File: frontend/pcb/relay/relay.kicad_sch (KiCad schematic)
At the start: 17 parts, among them J1 Conn_01x02, J2 Conn_01x02, J3 CONN_01X02, J4 Conn_01x02, K1 G6B-1114C-US5DC, Q3 BSS138, U2 DSN-MINI-360

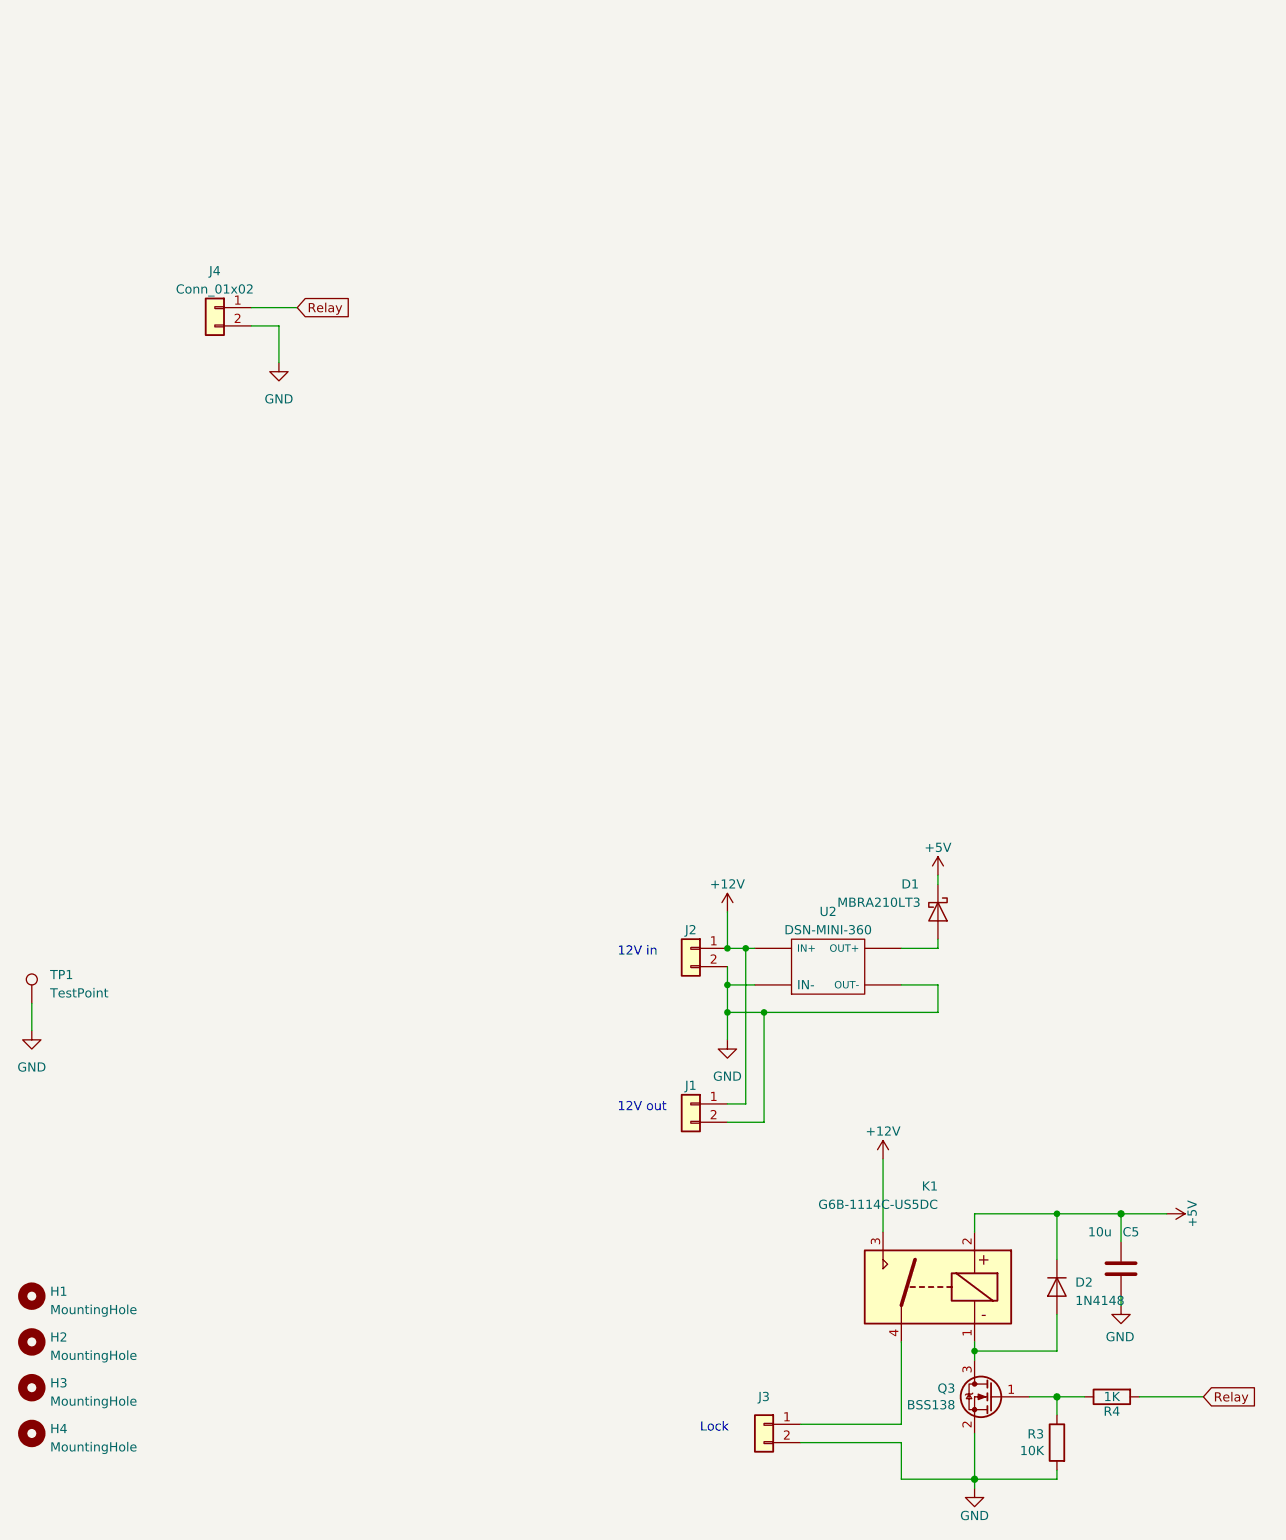
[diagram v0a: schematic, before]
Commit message: Finish relay board.
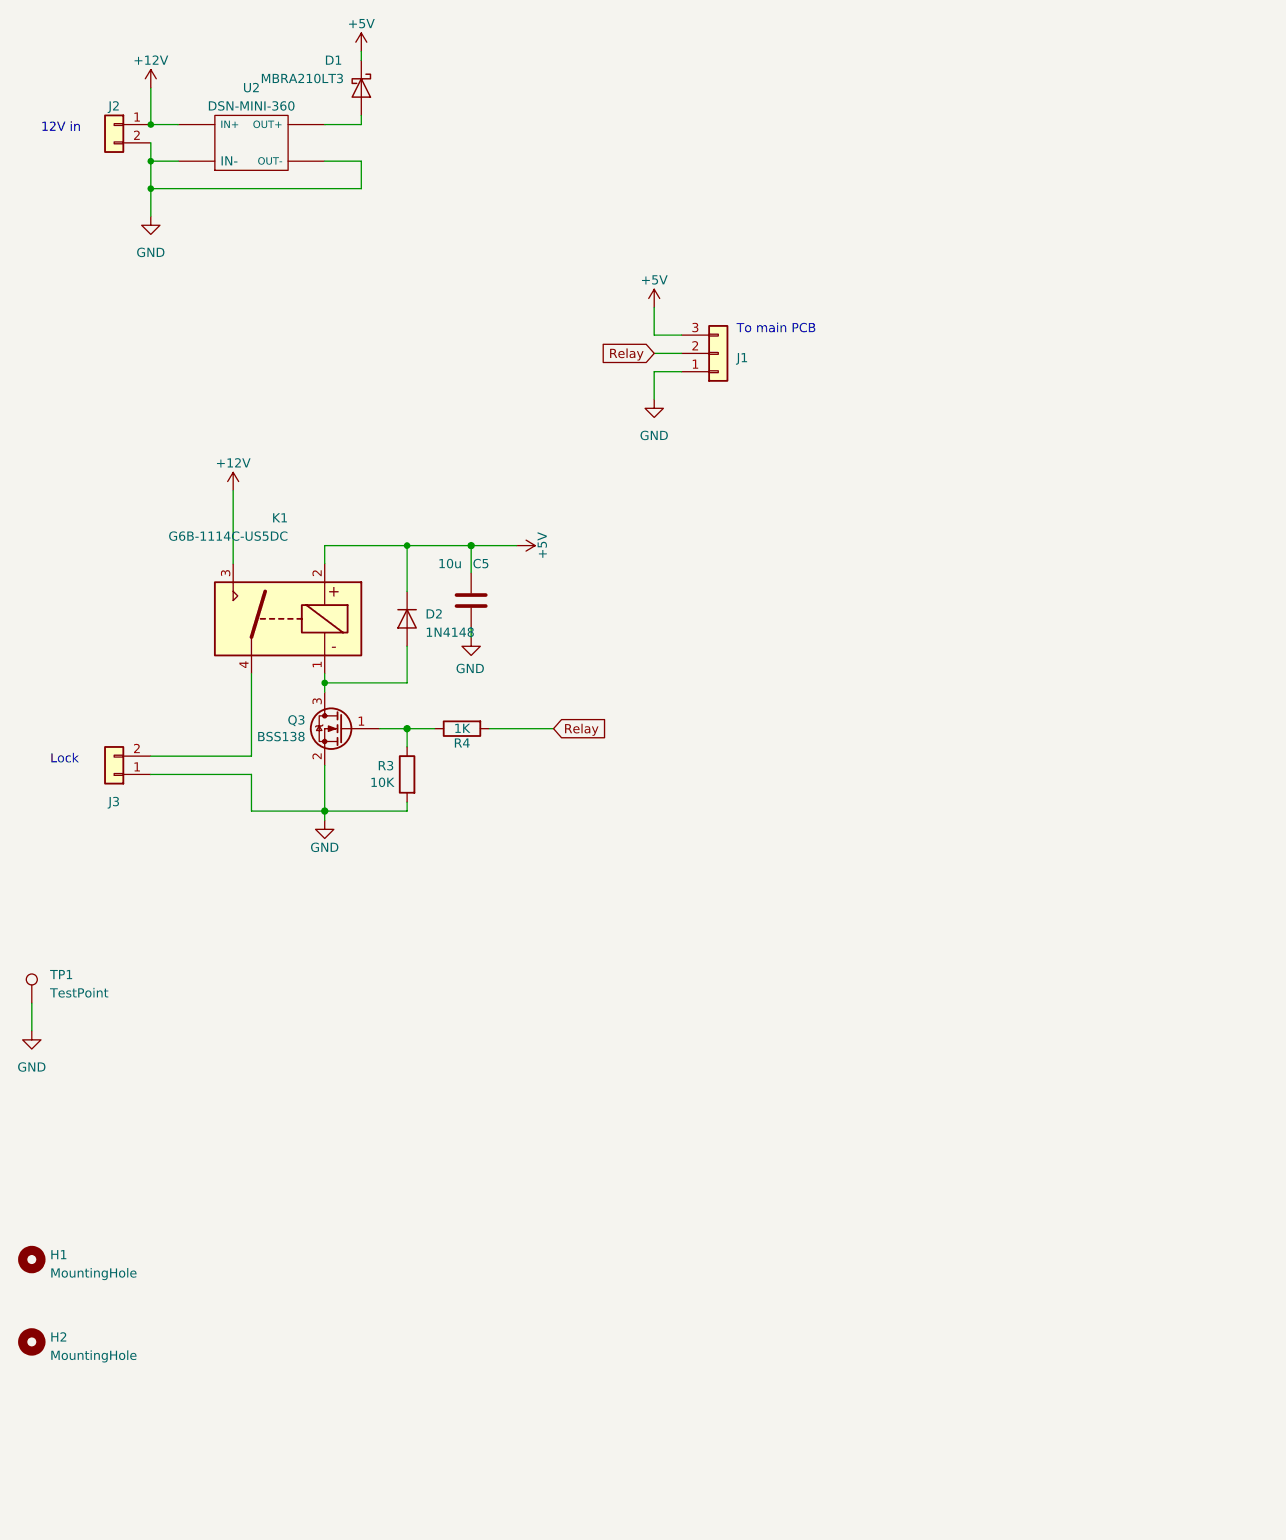
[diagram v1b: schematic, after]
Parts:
- removed H1, H3: MountingHole, MountingHole:MountingHole_3.2mm_M3, symbol Mechanical:MountingHole
- removed J1, J4: Conn_01x02, Connector_JST:JST_XH_B2B-XH-A_1x02_P2.50mm_Vertical, symbol Connector_Generic:Conn_01x02
- added J1: Conn_01x03, Connector_PinSocket_2.54mm:PinSocket_1x03_P2.54mm_Vertical, symbol Connector_Generic:Conn_01x03
- renumbered H4 to H1
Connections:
- net +5V: now also J1.3 (Pin_3)
- net GND: now also J3.1 (Pin_1), J1.1 (Pin_1); no longer J3.2 (Pin_2)
- net Relay: now also J1.2 (Pin_2)
- net at K1.4: now also J3.2 (Pin_2); no longer J3.1 (Pin_1)
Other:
- note added: "To main PCB"
- note removed: "12V out"
- moved on the sheet: C5, D1, D2, H1, J2, J3, K1, Q3, R3, R4, U2
